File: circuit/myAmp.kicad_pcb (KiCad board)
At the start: 2 copper layers, 100 x 100 mm, 48 parts, among them J1 JACK_MONO, J2 HOLE, J3 HOLE, J4 HOLE, J5 HOLE, Q1 J201, Q2 J201, U1 TPA3136D2

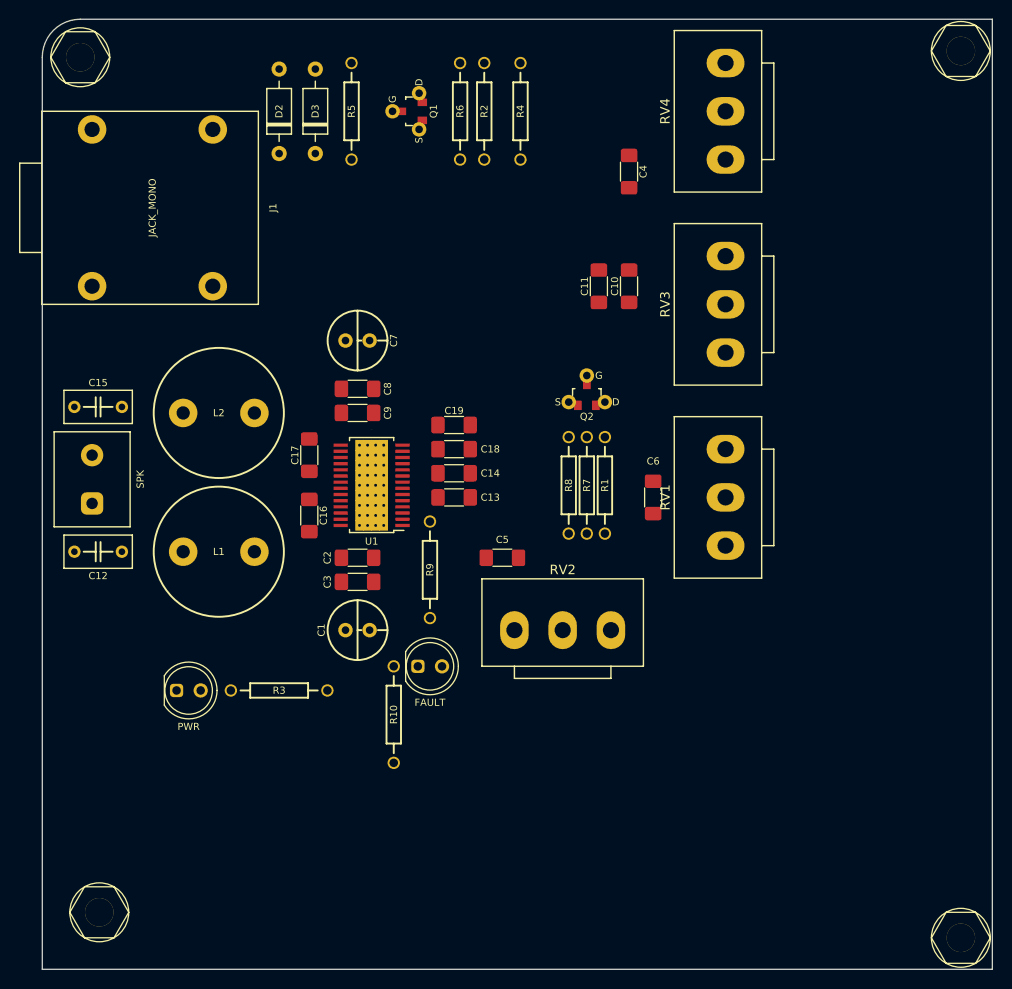
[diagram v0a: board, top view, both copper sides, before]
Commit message: more layout
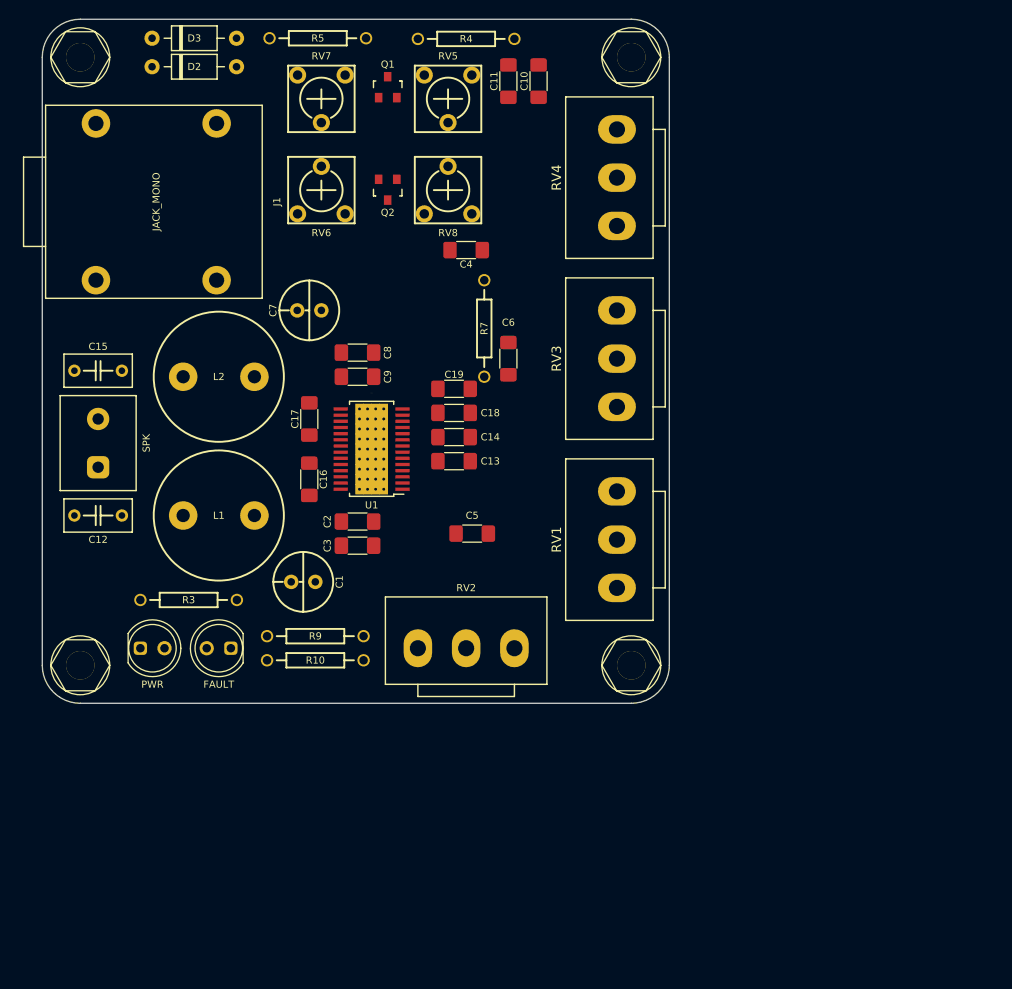
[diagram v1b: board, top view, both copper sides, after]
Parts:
- removed R1, R2: 6K8, myAmp:R_10MM
- removed R6, R8: 2K2, myAmp:R_10MM
- added RV5: 50K, myAmp:RPOT_RKT6V, F.Cu at (92.7, 55.9)
- added RV6: 50K, myAmp:RPOT_RKT6V, F.Cu at (79.4, 70.5)
- added RV7: 5K, myAmp:RPOT_RKT6V, F.Cu at (79.4, 55.9)
- added RV8: 50K, myAmp:RPOT_RKT6V, F.Cu at (92.7, 70.5)
- Q1, Q2: footprint myAmp:J201 -> myAmp:SOT-23
- moved J2 45.0 mm to (112.0, 118.0)
- moved J5 34.7 mm to (112.0, 54.0)
- moved Q2 30.1 mm to (86.4, 67.9), turned to 180 degrees
- moved J3 26.1 mm to (54.0, 118.0)
- moved C10 23.6 mm to (102.2, 56.5)
- moved C11 23.6 mm to (99.1, 56.5)
- moved D4 22.3 mm to (68.6, 116.2), turned to 180 degrees
- moved C6 21.1 mm to (99.1, 85.7)
- moved R7 19.7 mm to (96.5, 82.5), turned to 90 degrees
- moved C4 19.0 mm to (94.6, 74.3), turned to 180 degrees
- moved D3 14.9 mm to (66.0, 52.0), turned to 0 degrees
- moved R9 13.9 mm to (78.7, 114.9), turned to 0 degrees
- moved R3 13.5 mm to (65.4, 111.1)
- moved RV4 13.4 mm to (110.5, 66.7)
- moved RV3 12.8 mm to (110.5, 85.7)
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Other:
- board size 100 x 100 mm -> 66 x 72 mm
